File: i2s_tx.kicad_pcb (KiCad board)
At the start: 2 copper layers, 18 parts, among them IC1 AM26C31, IC2 AM26C31, IC3 AM26C31, J1 CONN_02x06, J2 CONN_02x06, J3 RJ45_Shielded, J4 RJ45_Shielded, J5 RJ45_Shielded, J6 CONN_01x02

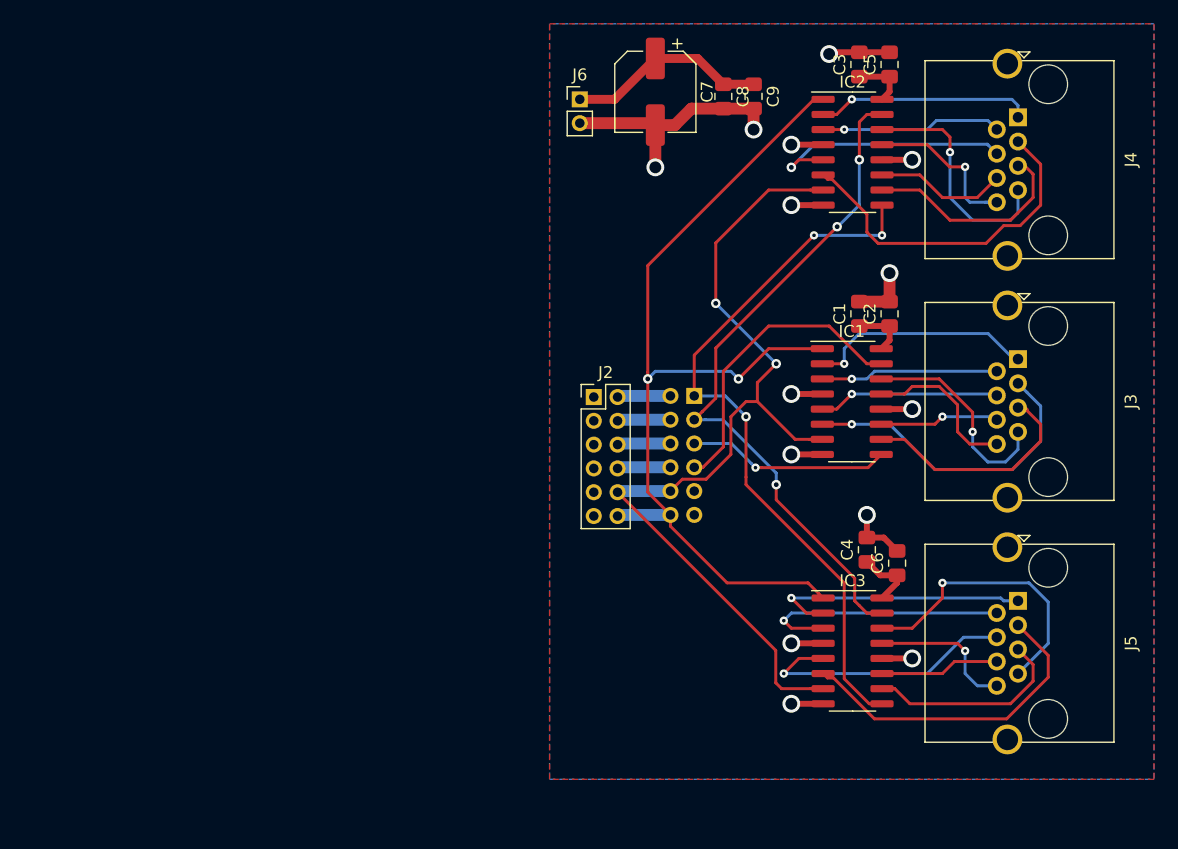
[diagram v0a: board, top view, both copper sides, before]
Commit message: -- update
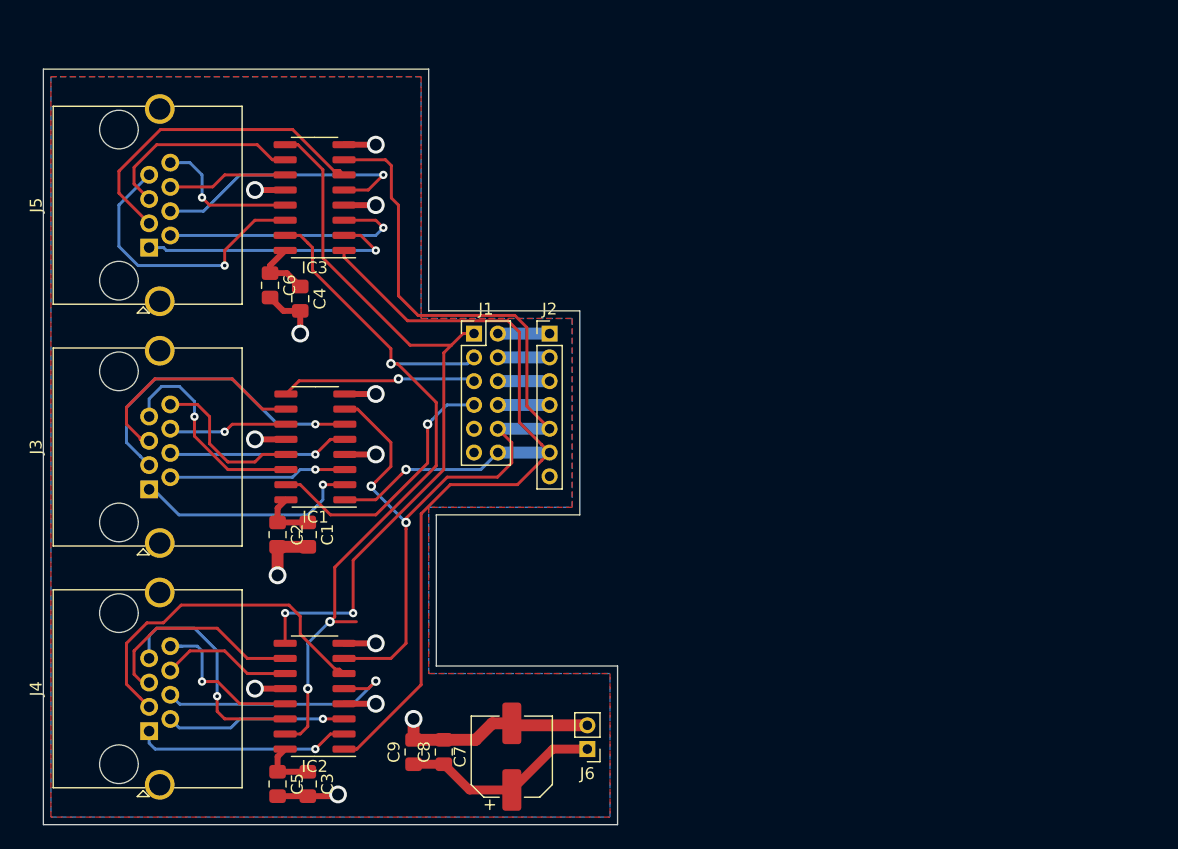
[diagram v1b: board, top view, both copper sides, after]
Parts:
- J1: moved to F.Cu
- J2: value CONN_02x06 -> CONN_01x07; footprint Connector_PinHeader_2.00mm:PinHeader_2x06_P2.00mm_Vertical -> Connector_PinHeader_2.00mm:PinHeader_1x07_P2.00mm_Vertical
- moved J4 89.4 mm to (36.2, 78.5), turned to 90 degrees
- moved C5 79.4 mm to (47.0, 82.9), turned to 270 degrees
- moved J5 78.8 mm to (36.2, 37.9), turned to 90 degrees
- moved C3 76.2 mm to (49.5, 82.9), turned to 270 degrees
- moved J3 73.8 mm to (36.2, 58.2), turned to 90 degrees
- moved IC2 64.3 mm to (50.1, 75.6), turned to 180 degrees
- moved C9 62.1 mm to (58.4, 80.3), turned to 90 degrees
- moved C8 59.9 mm to (61.0, 80.3), turned to 90 degrees
- moved IC3 59.1 mm to (50.1, 33.7), turned to 180 degrees
- moved C6 57.6 mm to (46.4, 41.0), turned to 270 degrees
- moved C7 57.2 mm to (66.7, 80.6), turned to 90 degrees
- moved C2 54.7 mm to (47.0, 62.0), turned to 270 degrees
- moved J6 54.6 mm to (73.0, 80.0), turned to 180 degrees
- moved C4 52.1 mm to (48.9, 42.2), turned to 270 degrees
- moved C1 49.9 mm to (49.5, 62.0), turned to 270 degrees
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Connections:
- J2 pad 1: Net-(J2-Pad1) -> I2S_IN_12
- J2 pad 2: I2S_IN_12 -> I2S_IN_34
- J2 pad 3: Net-(J2-Pad3) -> I2S_IN_56
- J2 pad 4: I2S_IN_34 -> I2S_IN_78
- J2 pad 5: Net-(J2-Pad5) -> I2S_SCLK
- J2 pad 6: I2S_IN_56 -> I2S_WS
- J2 pad 7: Net-(J2-Pad7) -> GND
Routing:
- net I2S_SCLK: track 76.3 -> 85.3 mm
- net I2S_OUT_34: track 58.0 -> 63.8 mm
- net I2S_WS: track 79.4 -> 85.0 mm, vias 2 -> 1
- net GND: track 59.0 -> 55.4 mm, vias 14 -> 13
- net I2S_OUT_78: track 25.7 -> 22.6 mm, vias 0 -> 1
- net I2S_OUT_12: track 60.5 -> 61.8 mm, vias 3 -> 2
- net I2S_OUT_56: track 17.0 -> 16.5 mm
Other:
- board outline added: 48.3 x 63.5 mm
